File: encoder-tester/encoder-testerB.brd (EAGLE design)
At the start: 121.9 x 64.4 mm, 12 parts, among them J3 POWER_JACKPTH_LOCK

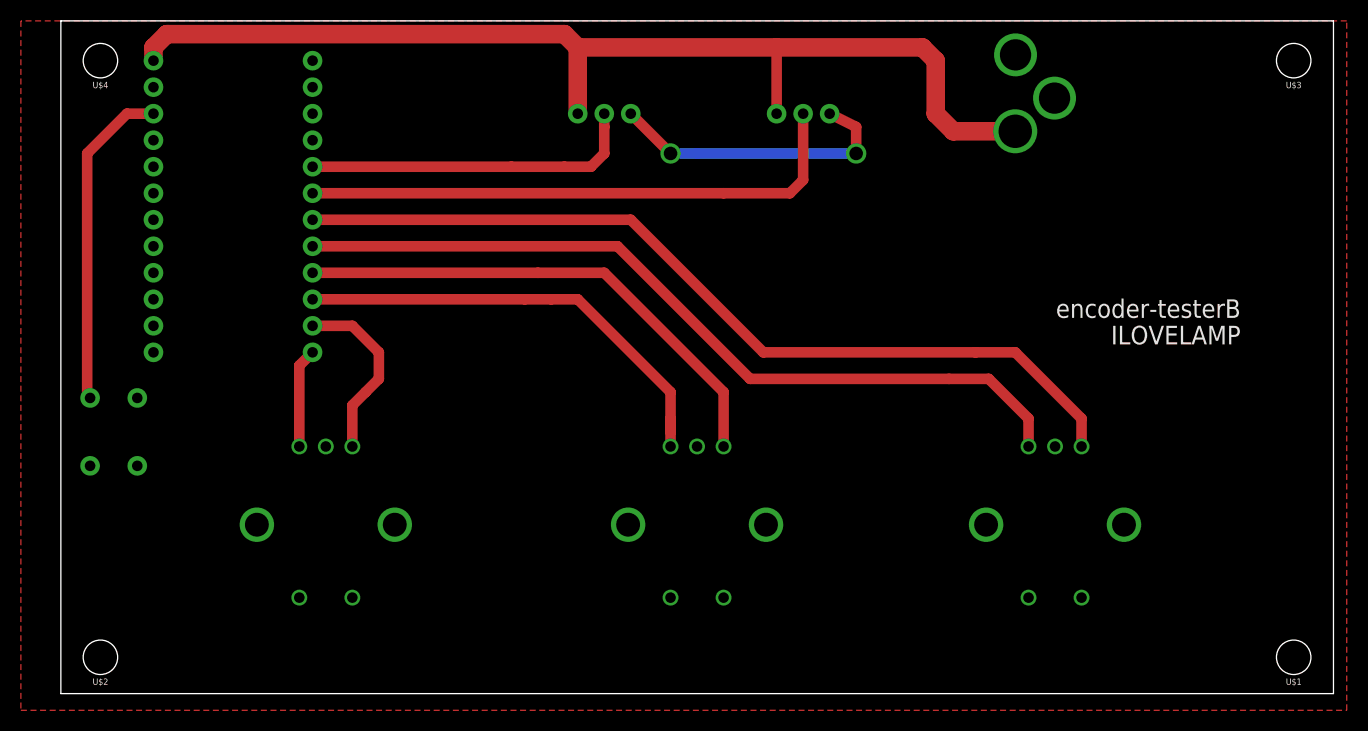
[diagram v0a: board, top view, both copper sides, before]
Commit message: update
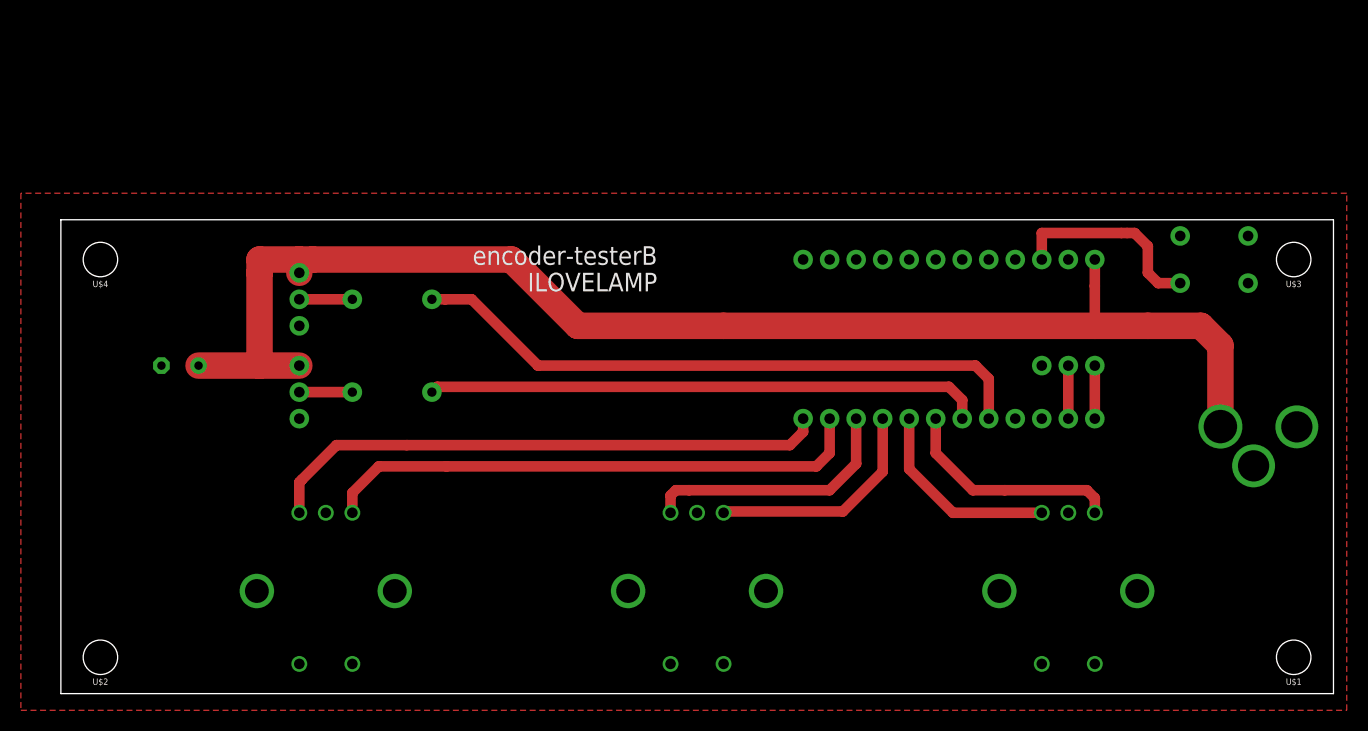
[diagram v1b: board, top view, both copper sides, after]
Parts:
- added C2: (no value), adafruit:E3,5-8
- added J4: (no value), SparkFun-Connectors:1X03
- added R1, R2: 1k, SparkFun-Resistors:AXIAL-0.3
- moved S4 106.7 mm to (110.5, 41.9), turned to 180 degrees
- moved B1 71.2 mm to (86.4, 34.3), turned to 90 degrees
- moved J3 53.9 mm to (125.0, 25.9), turned to 270 degrees
- moved J2 51.7 mm to (22.9, 31.8), turned to 270 degrees
- moved J1 30.7 mm to (22.9, 40.6), turned to 270 degrees
- moved U$3 19.1 mm to (118.1, 41.9)
- moved U$4 19.1 mm to (3.81, 41.9)
- moved S1 6.48 mm to (96.5, 10.2)
- moved S2 6.35 mm to (61.0, 10.2)
- moved S3 6.35 mm to (25.4, 10.2)
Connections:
- new net BUT3: S3.SW-
- new net N$1: J1.2, R1.P$2
- new net N$2: J2.2, R2.P$2
- new net N$3: B1.2, J4.2
- new net N$4: B1.1, J4.3
- net GND: now also C2.-, J4.1, S3.SW+
- net LED1: now also R1.P$1; no longer J1.2
- net LED2: now also R2.P$1; no longer J2.2
- net VIN: now also C2.+
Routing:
- net ENC1B: track 84.2 -> 21.7 mm
- net ENC1A: track 78.1 -> 19.4 mm
- net ENC3A: track 9.54 -> 54.4 mm
- net ENC3B: track 17.5 -> 52.5 mm
- net GND: track 28.5 -> 0.00 mm, vias 2 -> 0
- net LED1: track 32.3 -> 60.3 mm
- net ENC2B: track 49.3 -> 22.0 mm
- net VIN: track 103.9 -> 130.7 mm
- net ENC2A: track 44.4 -> 25.0 mm
- net RESET: track 31.5 -> 19.3 mm
- net N$2: track 0.00 -> 5.08 mm
- net N$1: track 0.00 -> 5.08 mm
- net N$4: track 0.00 -> 5.08 mm
- net N$3: track 0.00 -> 5.08 mm
- net LED2: track 53.9 -> 53.3 mm
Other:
- board size 121.9 x 64.4 mm -> 121.9 x 45.4 mm
